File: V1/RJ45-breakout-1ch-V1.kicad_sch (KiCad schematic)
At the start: 2 parts, among them J1 RJ45, J2 Screw_Terminal_01x04

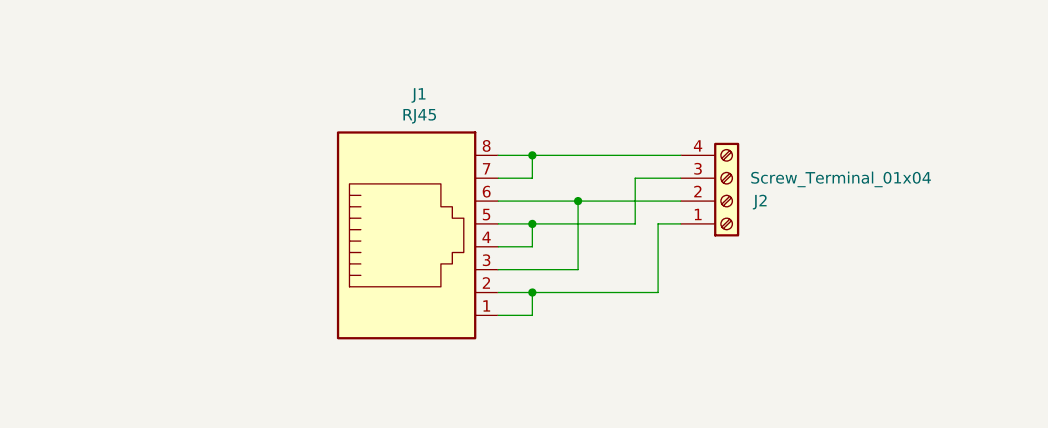
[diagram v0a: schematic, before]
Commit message: Footprint updated
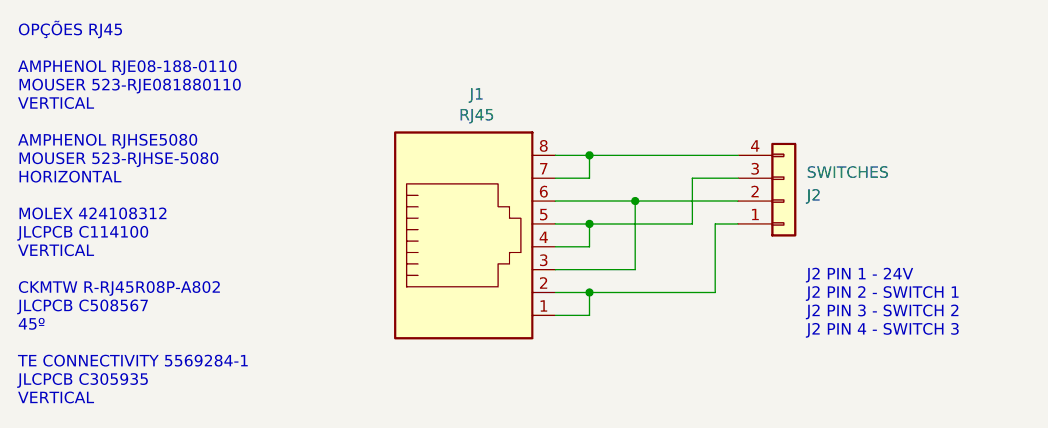
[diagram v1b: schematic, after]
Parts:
- removed J2: Screw_Terminal_01x04, Tales:TerminalBlock_Phoenix_MKDS-3-4-5.08_1x04_P5.08mm_Horizontal, symbol Connector:Screw_Terminal_01x04
- added J2: SWITCHES, symbol Connector_Generic:Conn_01x04
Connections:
- net at J1.1, J1.2: now also J2.1 (Pin_1)
- net at J1.3, J1.6: now also J2.2 (Pin_2)
- net at J1.4, J1.5: now also J2.3 (Pin_3)
- net at J1.7, J1.8: now also J2.4 (Pin_4)
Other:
- note added: "J2 PIN 1 - 24V J2 PIN 2 - SWITCH 1 J2 PIN 3 - SWITCH 2 J2 PIN 4 - SWITCH 3"
- note added: "OPÇÕES RJ45 AMPHENOL RJE08-188-0110 MOUSER 523-RJE081880110 VERTICAL AMPHENOL RJHSE5080 MOUSER 523-RJHSE-5080 HORIZONTAL MOLEX 424108312 JLCPCB C114100 VERTICAL CKMTW R-RJ45R08P-A802 JLCPCB C508567 45º TE CONNECTIVITY 5569284-1 JLCPCB C305935 VERTICAL"
- moved on the sheet: J1
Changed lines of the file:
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@@
     (rev "V1")
   )
-  (junction (at 146.05 99.06) (diameter 0) (color 0 0 0 0)
+  (junction (at 152.4 99.06) (diameter 0) (color 0 0 0 0)
   )
-  (junction (at 140.97 109.22) (diameter 0) (color 0 0 0 0)
+  (junction (at 147.32 109.22) (diameter 0) (color 0 0 0 0)
   )
-  (junction (at 140.97 93.98) (diameter 0) (color 0 0 0 0)
+  (junction (at 147.32 93.98) (diameter 0) (color 0 0 0 0)
   )
-  (junction (at 140.97 101.6) (diameter 0) (color 0 0 0 0)
+  (junction (at 147.32 101.6) (diameter 0) (color 0 0 0 0)
   )
-  (wire (pts (xy 140.97 96.52) (xy 140.97 93.98))
+  (wire (pts (xy 147.32 96.52) (xy 147.32 93.98))
     (stroke (width 0) (type default))
   )
-  (wire (pts (xy 137.16 104.14) (xy 140.97 104.14))
+  (wire (pts (xy 143.51 104.14) (xy 147.32 104.14))
     (stroke (width 0) (type default))
   )
-  (wire (pts (xy 154.94 101.6) (xy 157.48 101.6))
+  (wire (pts (xy 161.29 101.6) (xy 163.83 101.6))
     (stroke (width 0) (type default))
   )
-  (wire (pts (xy 140.97 93.98) (xy 137.16 93.98))
+  (wire (pts (xy 147.32 93.98) (xy 143.51 93.98))
     (stroke (width 0) (type default))
   )
-  (wire (pts (xy 140.97 111.76) (xy 140.97 109.22))
+  (wire (pts (xy 147.32 111.76) (xy 147.32 109.22))
     (stroke (width 0) (type default))
   )
-  (wire (pts (xy 152.4 101.6) (xy 152.4 96.52))
+  (wire (pts (xy 158.75 101.6) (xy 158.75 96.52))
     (stroke (width 0) (type default))
   )
-  (wire (pts (xy 137.16 96.52) (xy 140.97 96.52))
+  (wire (pts (xy 143.51 96.52) (xy 147.32 96.52))
     (stroke (width 0) (type default))
   )
-  (wire (pts (xy 140.97 101.6) (xy 137.16 101.6))
+  (wire (pts (xy 147.32 101.6) (xy 143.51 101.6))
     (stroke (width 0) (type default))
   )
-  (wire (pts (xy 140.97 109.22) (xy 137.16 109.22))
+  (wire (pts (xy 147.32 109.22) (xy 143.51 109.22))
     (stroke (width 0) (type default))
   )
-  (wire (pts (xy 146.05 99.06) (xy 137.16 99.06))
+  (wire (pts (xy 152.4 99.06) (xy 143.51 99.06))
     (stroke (width 0) (type default))
   )
-  (wire (pts (xy 146.05 99.06) (xy 157.48 99.06))
+  (wire (pts (xy 152.4 99.06) (xy 163.83 99.06))
     (stroke (width 0) (type default))
   )
-  (wire (pts (xy 140.97 101.6) (xy 152.4 101.6))
+  (wire (pts (xy 147.32 101.6) (xy 158.75 101.6))
     (stroke (width 0) (type default))
   )
-  (wire (pts (xy 146.05 106.68) (xy 146.05 99.06))
+  (wire (pts (xy 152.4 106.68) (xy 152.4 99.06))
     (stroke (width 0) (type default))
   )
-  (wire (pts (xy 140.97 93.98) (xy 157.48 93.98))
+  (wire (pts (xy 147.32 93.98) (xy 163.83 93.98))
     (stroke (width 0) (type default))
   )
-  (wire (pts (xy 137.16 106.68) (xy 146.05 106.68))
+  (wire (pts (xy 143.51 106.68) (xy 152.4 106.68))
     (stroke (width 0) (type default))
   )
-  (wire (pts (xy 154.94 109.22) (xy 154.94 101.6))
+  (wire (pts (xy 161.29 109.22) (xy 161.29 101.6))
     (stroke (width 0) (type default))
   )
-  (wire (pts (xy 137.16 111.76) (xy 140.97 111.76))
+  (wire (pts (xy 143.51 111.76) (xy 147.32 111.76))
     (stroke (width 0) (type default))
   )
-  (wire (pts (xy 140.97 104.14) (xy 140.97 101.6))
+  (wire (pts (xy 147.32 104.14) (xy 147.32 101.6))
     (stroke (width 0) (type default))
   )
-  (wire (pts (xy 152.4 96.52) (xy 157.48 96.52))
+  (wire (pts (xy 158.75 96.52) (xy 163.83 96.52))
     (stroke (width 0) (type default))
   )
-  (wire (pts (xy 140.97 109.22) (xy 154.94 109.22))
+  (wire (pts (xy 147.32 109.22) (xy 161.29 109.22))
     (stroke (width 0) (type default))
   )
-  (symbol (lib_id "Connector:Screw_Terminal_01x04") (at 162.56 99.06 0) (mirror x) (unit 1)
+  (text "OPÇÕES RJ45\n\nAMPHENOL RJE08-188-0110\nMOUSER 523-RJE081880110\nVERTICAL\n\nAMPHENOL RJHSE5080\nMOUSER 523-RJHSE-5080\nHORIZONTAL\n\nMOLEX 424108312\nJLCPCB C114100\nVERTICAL\n\nCKMTW R-RJ45R08P-A802\nJLCPCB C508567\n45º\n\nTE CONNECTIVITY 5569284-1\nJLCPCB C305935\nVERTICAL"
+    (at 83.82 121.92 0)
+    (effects (font (size 1.27 1.27)) (justify left bottom))
+  )
+  (text "J2 PIN 1 - 24V\nJ2 PIN 2 - SWITCH 1\nJ2 PIN 3 - SWITCH 2\nJ2 PIN 4 - SWITCH 3"
+    (at 171.45 114.3 0)
+    (effects (font (size 1.27 1.27)) (justify left bottom))
+  )
+  (symbol (lib_id "Connector:RJ45") (at 133.35 104.14 0) (unit 1)
     (in_bom yes) (on_board yes) (dnp no)
-    (property "Reference" "J2" (at 166.37 99.06 0)
+    (property "Reference" "J1" (at 134.7978 87.1982 0)
       (effects (font (size 1.27 1.27)))
     )
-    (property "Value" "Screw_Terminal_01x04" (at 175.26 96.52 0)
+    (property "Value" "RJ45" (at 134.7978 89.5096 0)
       (effects (font (size 1.27 1.27)))
     )
-    (property "Footprint" "Tales:TerminalBlock_Phoenix_MKDS-3-4-5.08_1x04_P5.08mm_Horizontal" (at 162.56 99.06 0)
+    (property "Footprint" "Tales:RJ45_Amphenol_RJHSE5080" (at 133.35 103.505 90)
       (effects (font (size 1.27 1.27)) hide)
     )
-    (property "Datasheet" "~" (at 162.56 99.06 0)
+    (property "Datasheet" "~" (at 133.35 103.505 90)
       (effects (font (size 1.27 1.27)) hide)
     )
-    (property "Case" "~" (at 162.56 99.06 0)
+    (property "Case" "~" (at 133.35 104.14 0)
       (effects (font (size 1.27 1.27)) hide)
     )
-    (property "Mfr" "Metaltex" (at 162.56 99.06 0)
+    (property "Mfr" "Amphenol" (at 133.35 104.14 0)
       (effects (font (size 1.27 1.27)) hide)
     )
-    (property "Mfr PN" "2x BR902V" (at 162.56 99.06 0)
+    (property "Mfr PN" "RJHSE-5080" (at 133.35 104.14 0)
       (effects (font (size 1.27 1.27)) hide)
     )
-    (property "Vendor" "Eletropecas" (at 162.56 99.06 0)
+    (property "Vendor" "Mouser" (at 133.35 104.14 0)
       (effects (font (size 1.27 1.27)) hide)
     )
-    (property "Vendor PN" "2x 29273" (at 162.56 99.06 0)
+    (property "Vendor PN" "523-RJHSE-5080" (at 133.35 104.14 0)
       (effects (font (size 1.27 1.27)) hide)
     )
-    (property "JLCPCB BOM" "~" (at 162.56 99.06 0)
+    (property "JLCPCB BOM" "~" (at 133.35 104.14 0)
       (effects (font (size 1.27 1.27)) hide)
     )
-    (property "LCSC Part" "~" (at 162.56 99.06 0)
-      (effects (font (size 1.27 1.27)) hide)
-    )
-    (pin "1")
-    (pin "2")
-    (pin "3")
-    (pin "4")
-    (instances
-      (project "RJ45-breakout-1ch-V1"
-        (path "/78f88cf6-751c-4e9b-ae75-fb8b6d44ff39"
-          (reference "J2") (unit 1)
-        )
-      )
-    )
-  )
-  (symbol (lib_id "Connector:RJ45") (at 127 104.14 0) (unit 1)
-    (in_bom yes) (on_board yes) (dnp no)
-    (property "Reference" "J1" (at 128.4478 87.1982 0)
-      (effects (font (size 1.27 1.27)))
-    )
-    (property "Value" "RJ45" (at 128.4478 89.5096 0)
-      (effects (font (size 1.27 1.27)))
-    )
-    (property "Footprint" "Tales:RJ45_Amphenol_RJHSE5080" (at 127 103.505 90)
-      (effects (font (size 1.27 1.27)) hide)
-    )
-    (property "Datasheet" "~" (at 127 103.505 90)
-      (effects (font (size 1.27 1.27)) hide)
-    )
-    (property "Case" "~" (at 127 104.14 0)
-      (effects (font (size 1.27 1.27)) hide)
-    )
-    (property "Mfr" "Amphenol" (at 127 104.14 0)
-      (effects (font (size 1.27 1.27)) hide)
-    )
-    (property "Mfr PN" "RJHSE-5080" (at 127 104.14 0)
-      (effects (font (size 1.27 1.27)) hide)
-    )
-    (property "Vendor" "Mouser" (at 127 104.14 0)
-      (effects (font (size 1.27 1.27)) hide)
-    )
-    (property "Vendor PN" "523-RJHSE-5080" (at 127 104.14 0)
-      (effects (font (size 1.27 1.27)) hide)
-    )
-    (property "JLCPCB BOM" "~" (at 127 104.14 0)
-      (effects (font (size 1.27 1.27)) hide)
-    )
-    (property "LCSC Part" "~" (at 127 104.14 0)
+    (property "LCSC Part" "~" (at 133.35 104.14 0)
       (effects (font (size 1.27 1.27)) hide)
     )
@@
         )
       )
+    )
+  )
+  (symbol (lib_id "Connector_Generic:Conn_01x04") (at 168.91 99.06 0) (mirror x) (unit 1)
+    (in_bom yes) (on_board yes) (dnp no)
+    (property "Reference" "J2" (at 171.45 98.425 0)
+      (effects (font (size 1.27 1.27)) (justify left))
+    )
+    (property "Value" "SWITCHES" (at 171.45 95.885 0)
+      (effects (font (size 1.27 1.27)) (justify left))
+    )
+    (property "Footprint" "" (at 168.91 99.06 0)
+      (effects (font (size 1.27 1.27)) hide)
+    )
+    (property "Datasheet" "~" (at 168.91 99.06 0)
+      (effects (font (size 1.27 1.27)) hide)
+    )
+    (pin "1")
+    (pin "2")
+    (pin "3")
+    (pin "4")
+    (instances
+      (project "RJ45-breakout-1ch-V1"
+        (path "/78f88cf6-751c-4e9b-ae75-fb8b6d44ff39"
+          (reference "J2") (unit 1)
+        )
+      )
